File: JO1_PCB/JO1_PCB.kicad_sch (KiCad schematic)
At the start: 23 parts, among them J1 CN8, J10 MCP2515_SPI, J11 MCP2515_CAN, J12 LM2596_3.3V, J13 LM2596_5V, J14 7.4V, J2 CN7, J3 CN9, J4 CN10, J5 DC_MOTOR, J6 ESC_MOTOR, J7 ESC_PWM, J8 MPU6050, J9 TJA1051, M1 SERVO, U1 NRF24L01

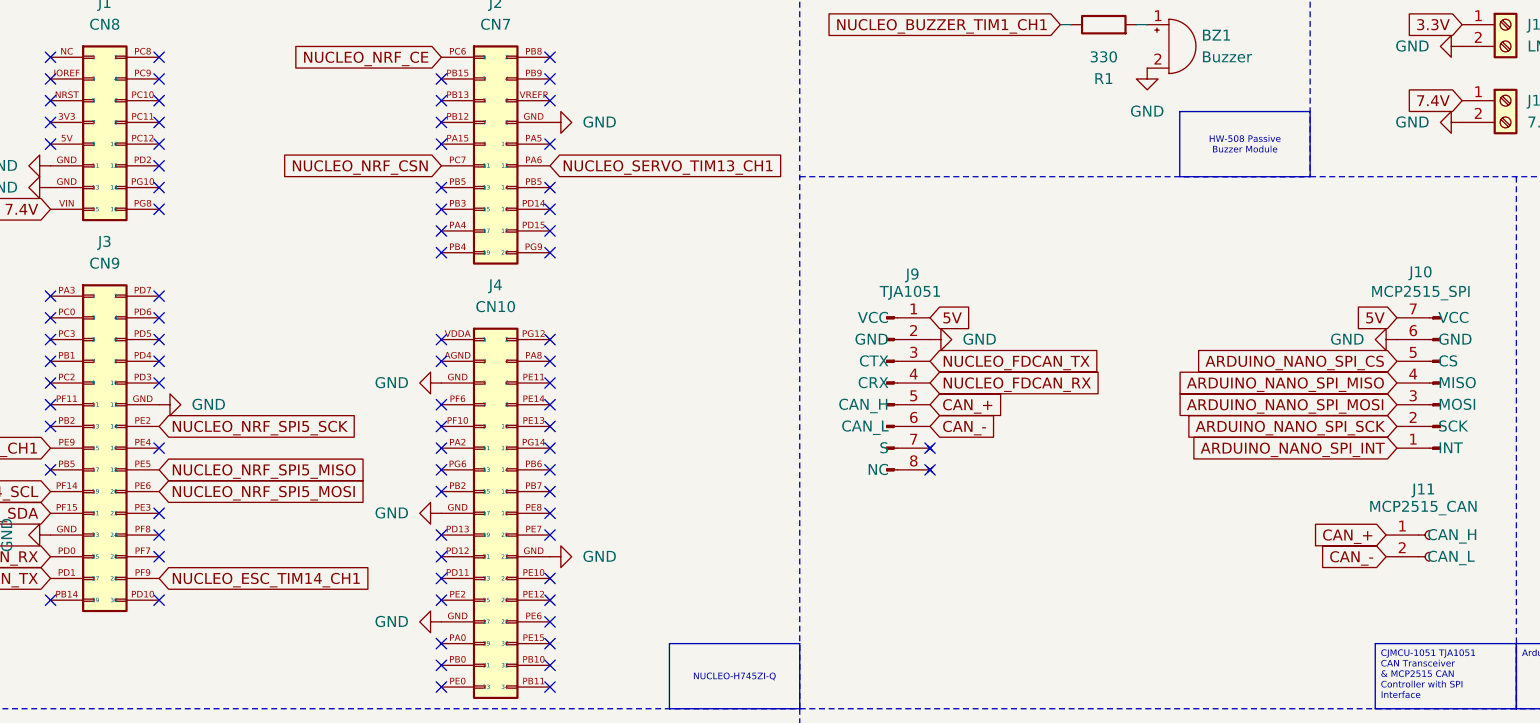
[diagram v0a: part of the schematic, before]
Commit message: Routed PCB
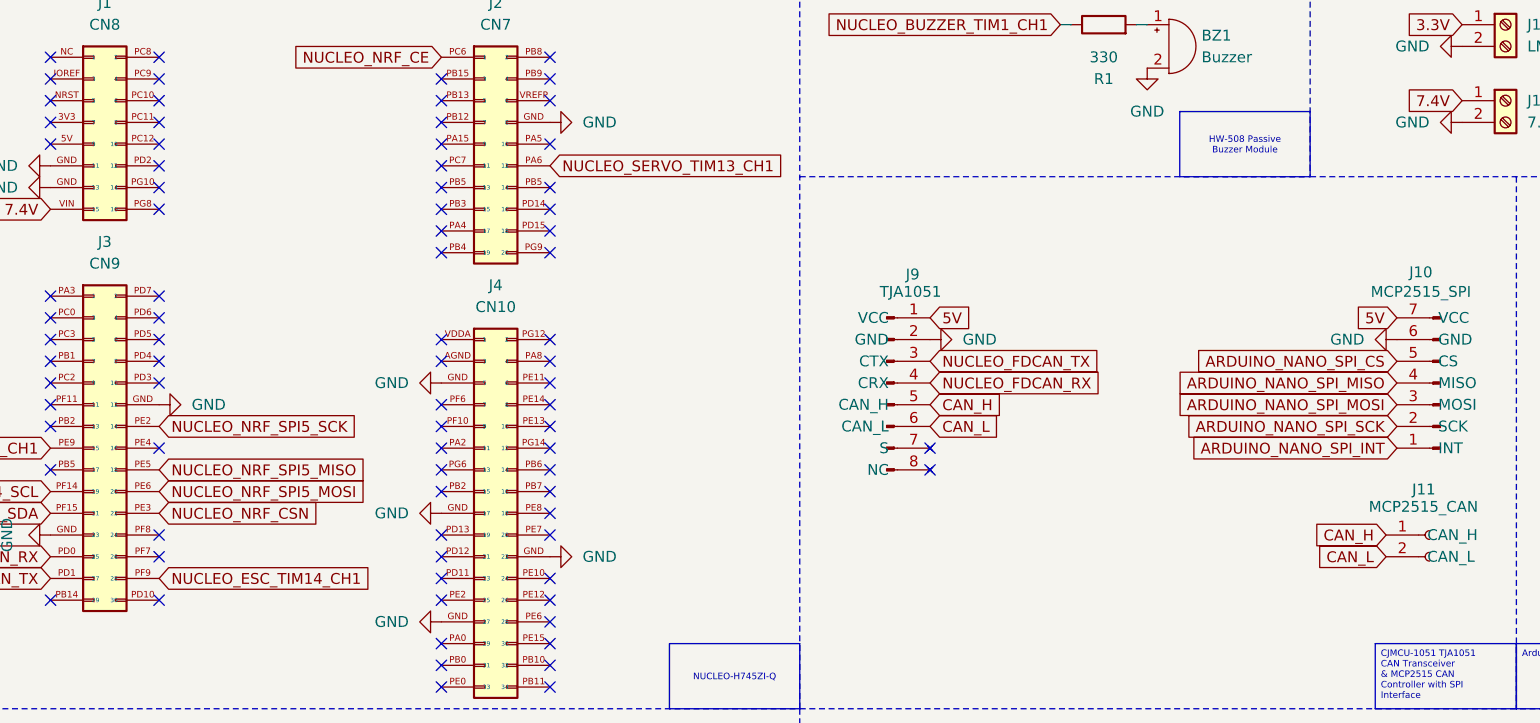
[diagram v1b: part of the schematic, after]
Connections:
- net NUCLEO_NRF_CSN: now also J3.PE3 (22); no longer J2.PC7 (11)
- net CAN_+ renamed CAN_H
- net CAN_- renamed CAN_L
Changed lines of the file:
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@@
+	)
+	(no_connect
+		(at 87.63 34.29)
 	)
 	(no_connect
@@
 	)
 	(no_connect
-		(at 54.61 74.93)
-	)
-	(no_connect
 		(at 54.61 77.47)
 	)
@@
 	)
 	(no_connect
+		(at 54.61 49.53)
+	)
+	(no_connect
 		(at 274.32 76.2)
 	)
@@
 	(no_connect
 		(at 54.61 54.61)
-	)
-	(no_connect
-		(at 54.61 49.53)
 	)
 	(no_connect
@@
 		)
 	)
+	(global_label "NUCLEO_NRF_CSN"
+		(shape input)
+		(at 54.61 74.93 0)
+		(fields_autoplaced yes)
+		(effects
+			(font
+				(size 1.27 1.27)
+			)
+			(justify left)
+		)
+		(property "Intersheetrefs" "${INTERSHEET_REFS}"
+			(at 74.4681 74.93 0)
+			(effects
+				(font
+					(size 1.27 1.27)
+				)
+				(justify left)
+				(hide yes)
+			)
+		)
+	)
 	(global_label "3.3V"
 		(shape input)
@@
 		)
 	)
-	(global_label "CAN_+"
+	(global_label "CAN_H"
 		(shape input)
 		(at 198.12 77.47 180)
@@
 		)
 		(property "Intersheetrefs" "${INTERSHEET_REFS}"
-			(at 188.9057 77.47 0)
+			(at 189.1476 77.47 0)
 			(effects
 				(font
@@
 		)
 	)
-	(global_label "CAN_-"
+	(global_label "CAN_L"
 		(shape input)
 		(at 144.78 64.77 0)
@@
 		)
 		(property "Intersheetrefs" "${INTERSHEET_REFS}"
-			(at 153.9943 64.77 0)
+			(at 153.45 64.77 0)
 			(effects
 				(font
@@
 		)
 	)
-	(global_label "CAN_+"
+	(global_label "CAN_H"
 		(shape input)
 		(at 144.78 62.23 0)
@@
 		)
 		(property "Intersheetrefs" "${INTERSHEET_REFS}"
-			(at 153.9943 62.23 0)
+			(at 153.7524 62.23 0)
 			(effects
 				(font
@@
 		)
 	)
-	(global_label "NUCLEO_NRF_CSN"
-		(shape input)
-		(at 87.63 34.29 180)
-		(fields_autoplaced yes)
-		(effects
-			(font
-				(size 1.27 1.27)
-			)
-			(justify right)
-		)
-		(property "Intersheetrefs" "${INTERSHEET_REFS}"
-			(at 67.7719 34.29 0)
-			(effects
-				(font
-					(size 1.27 1.27)
-				)
-				(justify right)
-				(hide yes)
-			)
-		)
-	)
 	(global_label "5V"
 		(shape input)
@@
 		)
 	)
-	(global_label "CAN_-"
+	(global_label "CAN_L"
 		(shape input)
 		(at 198.12 80.01 180)
@@
 		)
 		(property "Intersheetrefs" "${INTERSHEET_REFS}"
-			(at 188.9057 80.01 0)
-			(effects
-				(font
+			(at 189.45 80.01 0)
+			(effects
+				(font
